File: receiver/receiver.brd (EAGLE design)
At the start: 100 x 80 mm, 9 parts, among them P1 PROMICRO_HEADER, P2 PROMICRO_HEADER, U1 CORE51822B, U2 3.3

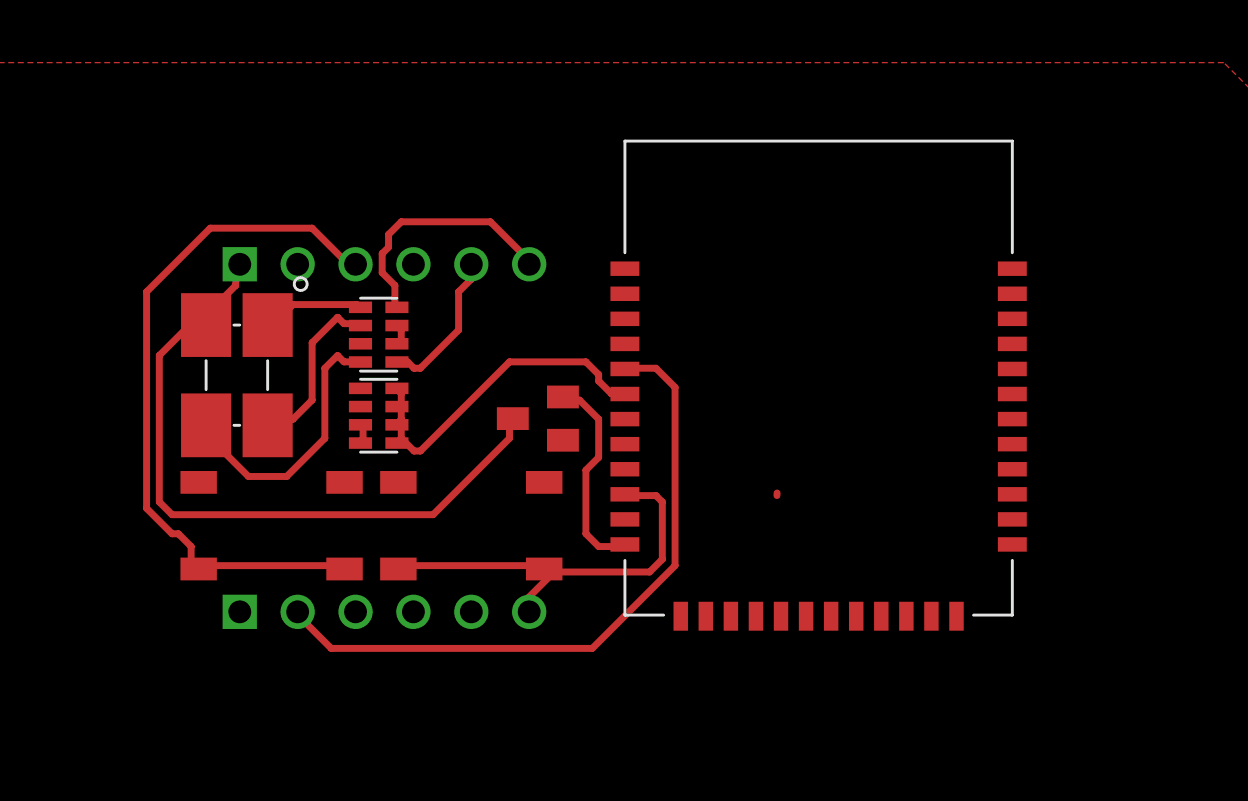
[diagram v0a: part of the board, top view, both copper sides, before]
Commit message: update board
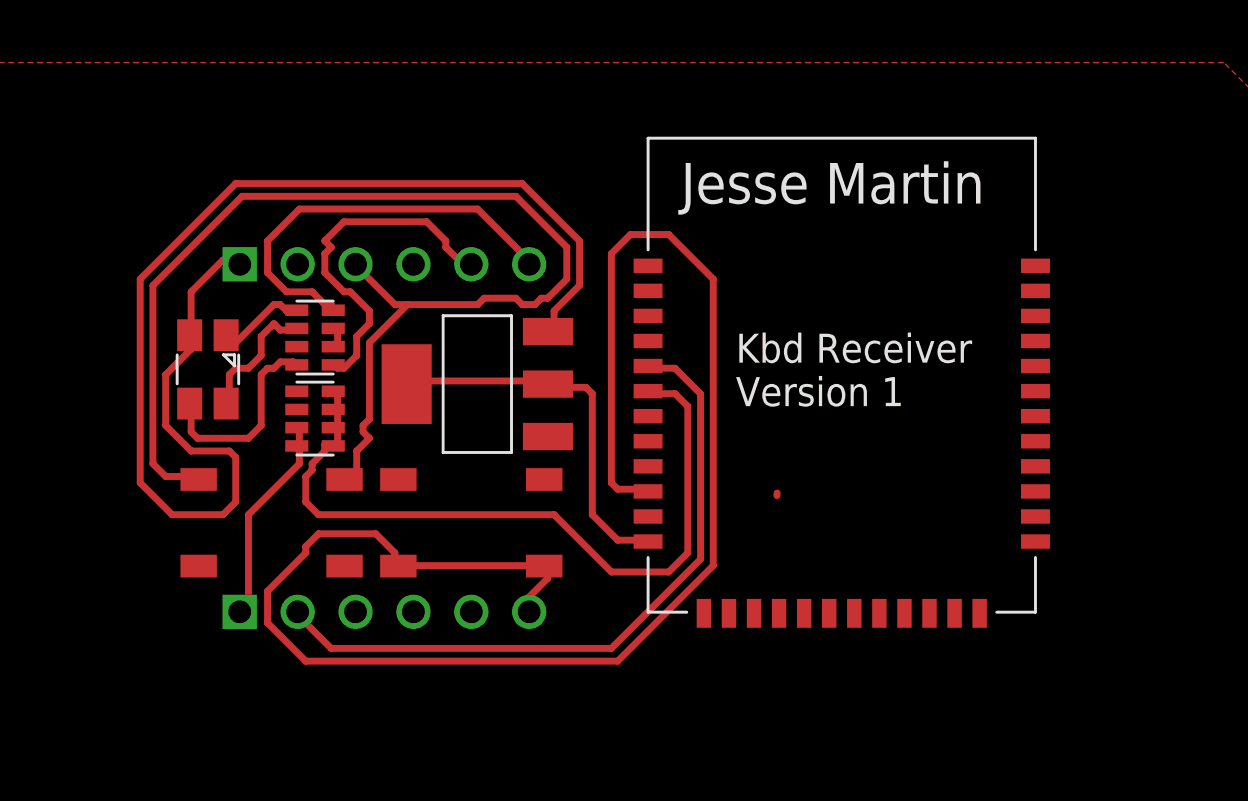
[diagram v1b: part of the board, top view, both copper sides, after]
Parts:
- U2: value 3.3 -> AZ1117IH; device adafruit:SOT23 -> az1117ih:AZ1117IH
- moved U2 3.06 mm to (56.1, 55.7)
- moved RA1 2.80 mm to (49.0, 57.8)
- moved RA2 2.80 mm to (49.0, 54.2)
- moved D1 1.30 mm to (44.3, 56.4)
- moved U1 1.02 mm to (72.1, 56.1)
- moved B1 0.13 mm to (55.9, 49.7)
- moved B2 0.13 mm to (47.1, 49.7), turned to 180 degrees
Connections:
- net GND: now also U2.ADJ/GND; no longer U2.1
- net VCC: now also U2.OUTPUT, U2.VOUT; no longer U2.2
- net VIN: now also U2.INPUT; no longer U2.3
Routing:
- net PAIR: track 18.9 -> 70.0 mm
- net VIN: track 30.4 -> 55.4 mm
- net RESET: track 31.1 -> 52.1 mm
- net TXO-DIV: track 15.4 -> 33.1 mm
- net LED-B: track 6.63 -> 15.6 mm
- net TXO: track 0.92 -> 9.30 mm
- net VCC: track 9.23 -> 16.8 mm
- net LED-R: track 10.8 -> 18.2 mm
- net N$14: track 12.1 -> 8.75 mm
- net N$10: track 7.64 -> 5.83 mm
- net RXI: track 29.2 -> 30.1 mm
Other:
- board text added: "Jesse Martin"
- board text added: "Kbd Receiver Version 1"
